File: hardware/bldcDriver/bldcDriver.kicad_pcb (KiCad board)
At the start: 4 copper layers, 89.8 x 41.5 mm, 187 parts, among them CN1 MR30PW-F, CN2 MR30PW-F, J1 Conn_01x02, J2 Conn_01x06, J3 Conn_01x06, J4 Conn_01x03, J5 Conn_01x06, Q1 KNY3406C, Q10 KNY3406C, Q11 KNY3406C, Q12 KNY3406C, Q13 PMOS, Q14 S8050, Q2 KNY3406C, Q3 KNY3406C, Q4 KNY3406C, Q5 KNY3406C, Q6 KNY3406C, Q7 KNY3406C, Q8 KNY3406C, Q9 KNY3406C, U1 FD6288T, U10 AMS1117, U11 FD6288T, U2 STM32G431RBTx, U3 TPS5430DDA, U4 MPU-6050, U6 TLV9062xD, U7 MT3608, U8 TLV9062xD, U9 TLV9062xD, Y1 25MHz

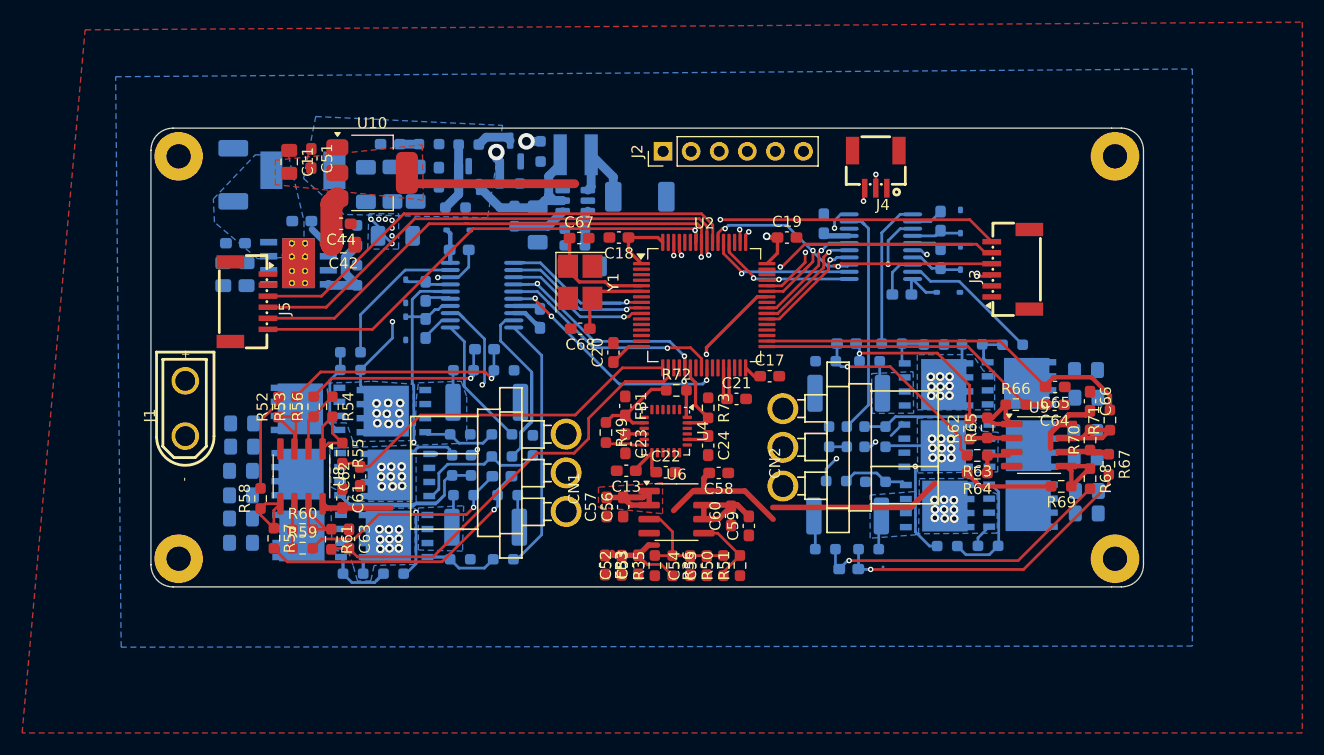
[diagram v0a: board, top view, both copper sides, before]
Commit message: update driver pcn
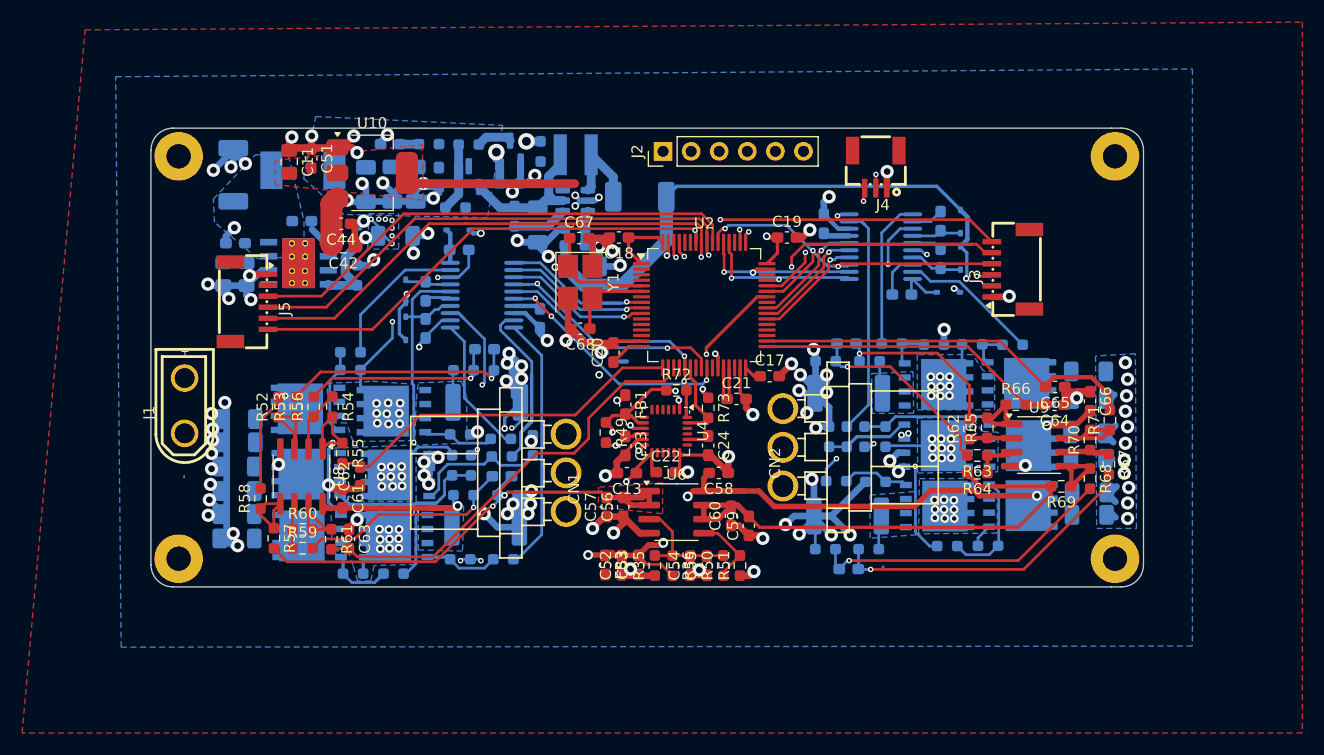
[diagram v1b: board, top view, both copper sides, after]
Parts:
- C29, C31, C33, C34, C35, C37, C39, C40, C41, C43, C45, C46: footprint Capacitor_SMD:C_0805_2012Metric_Pad1.18x1.45mm_HandSolder -> Capacitor_SMD:C_1206_3216Metric_Pad1.33x1.80mm_HandSolder
- moved C29 0.53 mm to (40.3, 57.0)
- moved C33 0.53 mm to (40.3, 59.1)
- moved C35 0.53 mm to (40.2, 65.6)
- moved C39 0.53 mm to (40.2, 67.8)
- moved C41 0.53 mm to (40.2, 61.3)
- moved C45 0.53 mm to (40.2, 63.5)
- moved R18 0.42 mm to (64.1, 58.8)
- moved C31 0.26 mm to (117.3, 52.7)
- moved C43 0.26 mm to (117.2, 58.3)
- moved C34 0.26 mm to (117.3, 55.2)
- moved C37 0.26 mm to (117.3, 65.7)
- moved C40 0.26 mm to (117.3, 63.6)
- moved C46 0.26 mm to (117.2, 60.6)
- moved J1 0.26 mm to (35.5, 55.8)
- moved C13 0.22 mm to (75.5, 61.9)
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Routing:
- net GNDPWR: track 9.57 -> 208.5 mm, vias 0 -> 88
- net GNDD: track 3.32 -> 114.3 mm, vias 7 -> 41
- net +12V: track 0.00 -> 78.2 mm, vias 0 -> 5
- net /OP_VCC: track 49.7 -> 95.7 mm, vias 0 -> 6
- net /VREF_OP1: track 18.7 -> 52.5 mm, vias 0 -> 2
- net /inverter/1SH_W: track 21.7 -> 51.9 mm, vias 9 -> 11
- net /VREF_OP2: track 16.8 -> 46.5 mm
- net Net-(U4-VDD): track 12.7 -> 24.7 mm, vias 0 -> 4
- net +3V3: track 35.8 -> 40.3 mm, vias 1 -> 3
- net Net-(Q12-G): track 3.54 -> 7.70 mm
- net /TIM8_CH1N: track 12.9 -> 14.1 mm
- net /TIM8_CH2N: track 13.3 -> 14.0 mm
- net /MPU_INT: track 3.55 -> 4.14 mm, vias 0 -> 2
- net /SPI1_MISO: track 88.7 -> 89.3 mm
- added copper zone on B.Cu, net GNDPWR
